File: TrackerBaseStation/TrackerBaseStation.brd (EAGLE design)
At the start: 14 x 38.1 mm, 24 parts, among them J1 DF12A3.0-14DS, Q1 16MHz, U1 ATMEGA8U2MU, U2 RCLAMP0502A, U3 NRF24L01NOPAD, U4 BD2425NNRF0404, X1 USB-LEG

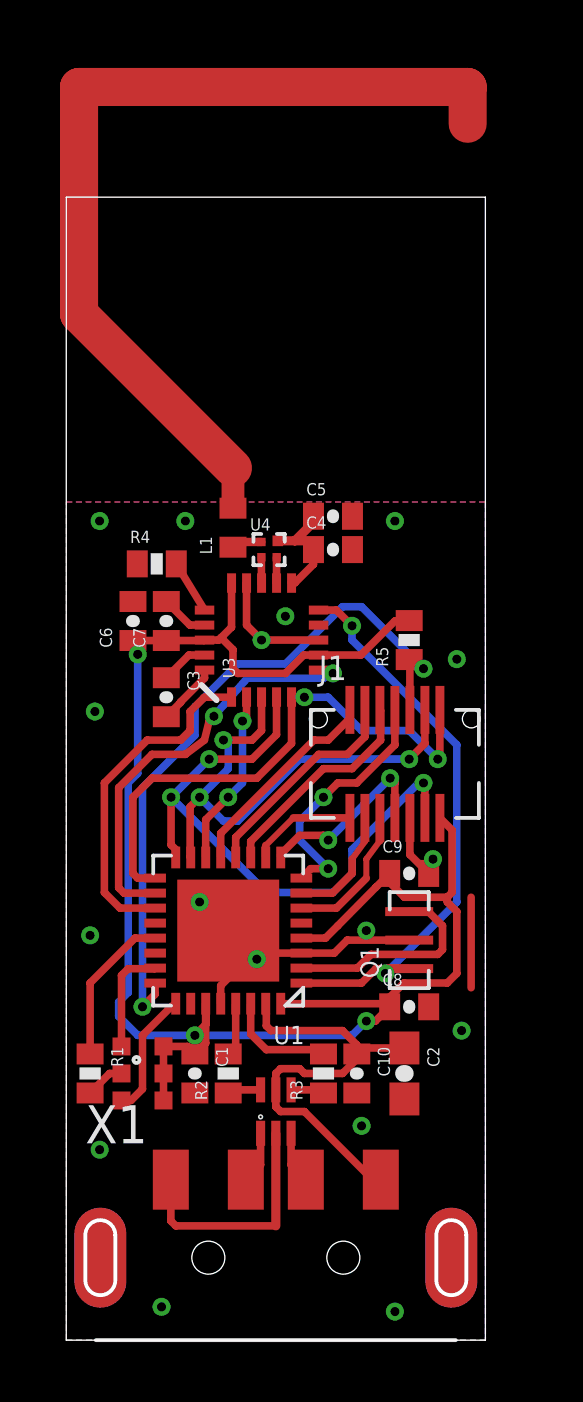
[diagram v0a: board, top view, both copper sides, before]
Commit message: silkscreen
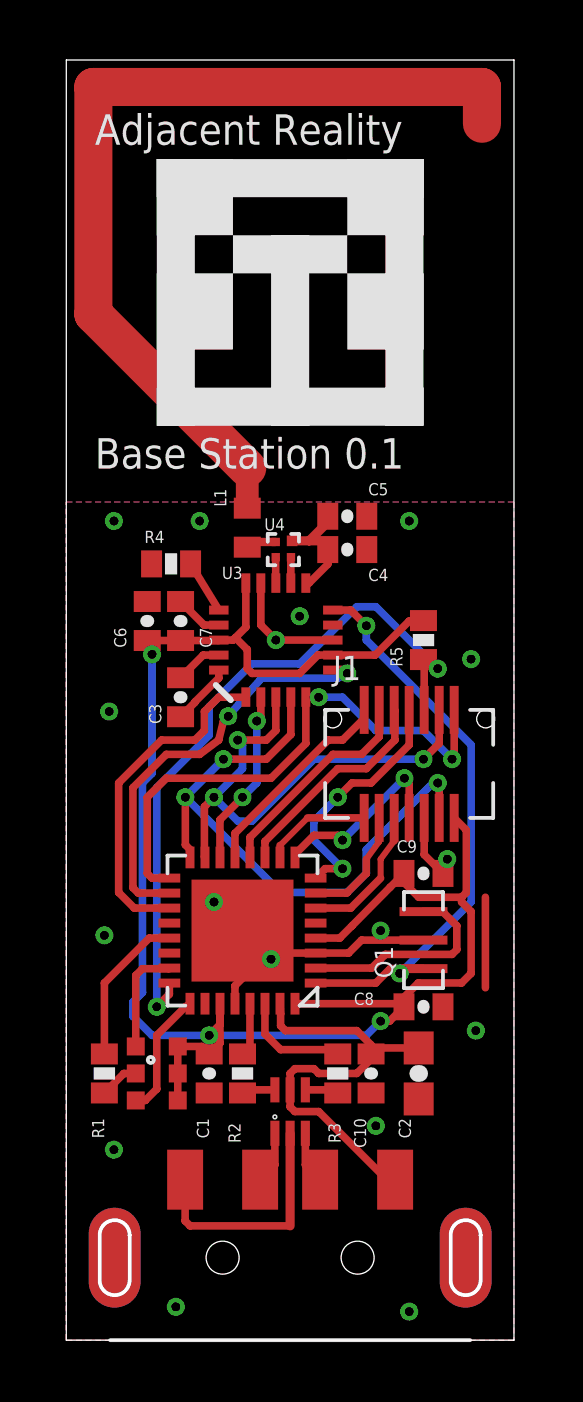
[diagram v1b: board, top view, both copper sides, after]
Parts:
- added U$1: (no value), adjacent-reality:ADJACENTREALITY-LOGO-0.35
- added U$2: (no value), SparkFun-Aesthetics:OSHW-LOGO-M
- moved C1 0.48 mm to (4.76, 8.89)
- moved C10 0.48 mm to (10.2, 8.89)
- moved C2 0.48 mm to (11.7, 8.89)
- moved C4 0.48 mm to (9.37, 26.4)
- moved C5 0.48 mm to (9.37, 27.5)
- moved C8 0.48 mm to (11.9, 11.1)
- moved C9 0.48 mm to (11.9, 15.6)
- moved J1 0.48 mm to (11.4, 19.2)
- moved Q1 0.48 mm to (11.9, 13.3)
- moved R2 0.48 mm to (5.87, 8.89)
- moved R3 0.48 mm to (9.05, 8.89)
- moved R4 0.48 mm to (3.49, 25.9)
- moved R5 0.48 mm to (11.9, 23.3)
- moved U1 0.48 mm to (5.87, 13.7)
- moved U3 0.48 mm to (6.99, 23.3)
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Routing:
- net ANT: track 0.00 -> 30.3 mm
- net N$26: track 13.0 -> 0.00 mm
- net N$25: track 7.57 -> 0.00 mm
- net N$18: track 7.26 -> 0.00 mm
- net N$27: track 1.23 -> 0.00 mm
- net N$14: track 1.13 -> 0.00 mm
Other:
- board size 14 x 38.1 mm -> 14.9 x 42.7 mm
- board text added: "Adjacent Reality"
- board text added: "Base Station 0.1"
- board text added: "Creative Commons By"
- board text added: "Nirav Patel <nrp@eclecti.cc>"
- board text added: "http://adjacentreality.org"
